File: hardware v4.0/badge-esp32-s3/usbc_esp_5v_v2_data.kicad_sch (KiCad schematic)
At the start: 22 parts, among them J2 Connector, USB-TYPE-C-16P, Q10 AO3424, U11 SY6288F1ABC, U12 SY6288F1ABC, U8 TUSB321AIRWBR

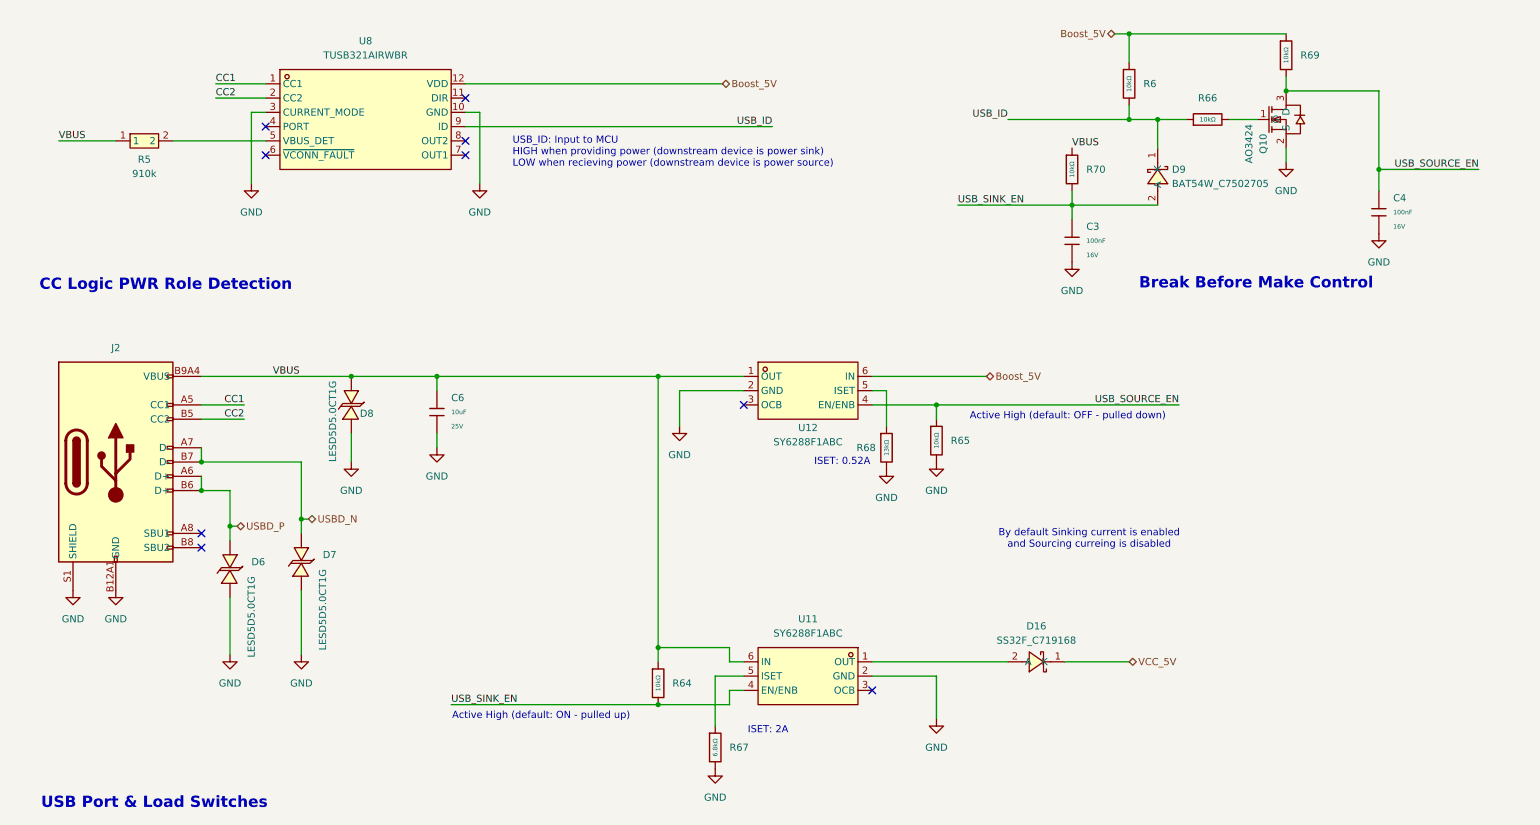
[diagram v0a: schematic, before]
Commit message: finished schematics and layout
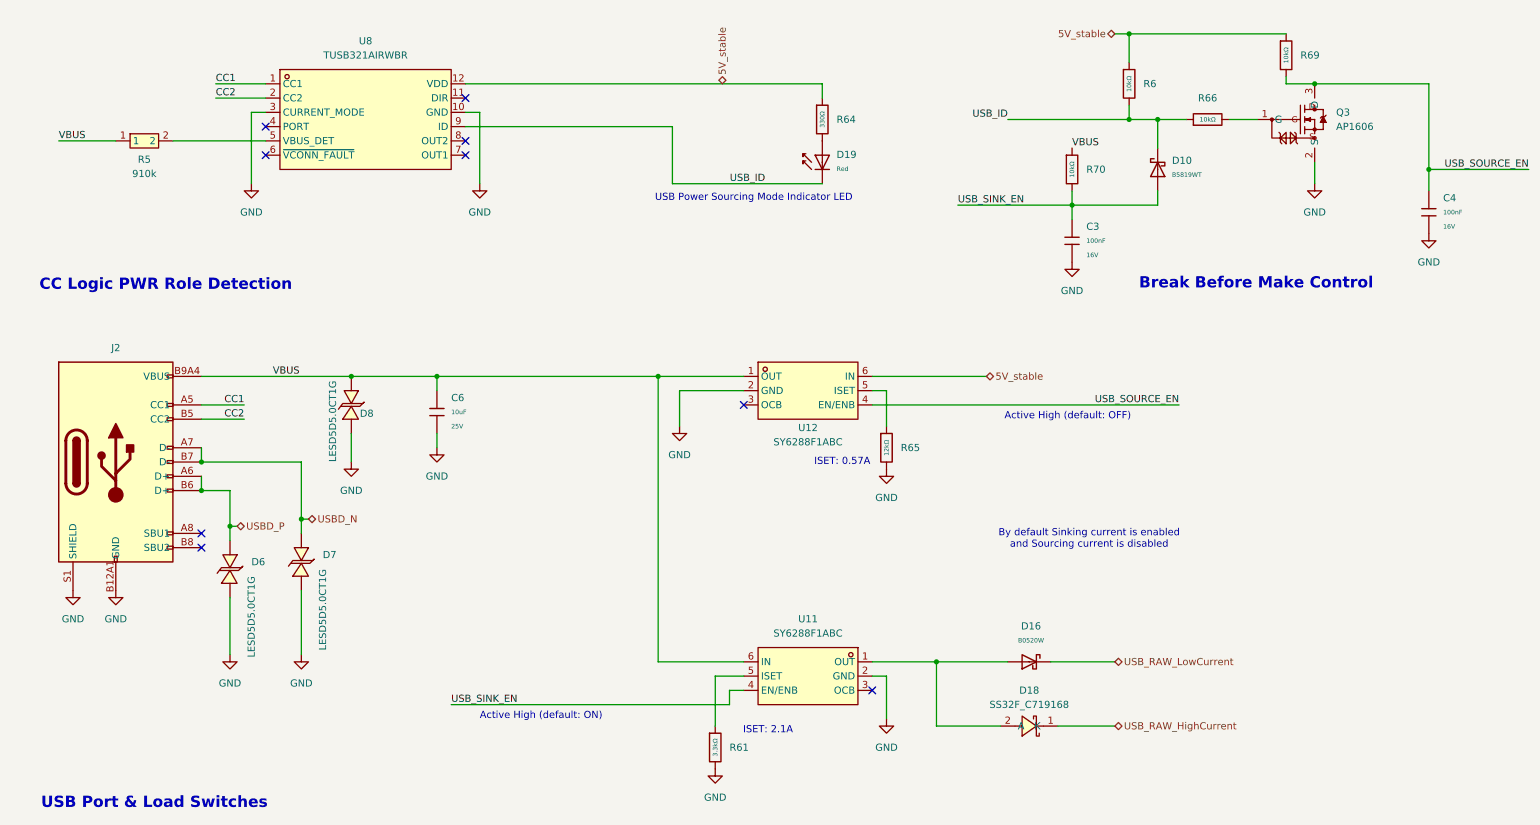
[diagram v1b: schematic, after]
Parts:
- removed D16: SS32F_C719168, lcsc-lib:SMAF_L3.5-W2.6-LS4.7-RD, symbol lcsc-lib:SS32F_C719168
- removed D9: BAT54W_C7502705, lcsc-lib:SOD-123_L2.7-W1.6-LS3.7-RD, symbol lcsc-lib:BAT54W_C7502705
- removed Q10: AO3424, lcsc-lib:SC-59-3_L2.9-W1.6-P0.95-LS2.9-BR, symbol lcsc-lib:AO3424
- removed R64, R65: 10kΩ, PCM_JLCPCB:R_0402, symbol PCM_JLCPCB-Resistors:0402,10kΩ
- removed R67: 6.8kΩ, PCM_JLCPCB:R_0402, symbol PCM_JLCPCB-Resistors:0402,6.8kΩ
- removed R68: 13kΩ, PCM_JLCPCB:R_0603, symbol PCM_JLCPCB-Resistors:0603,13kΩ
- added D10: B5819WT, PCM_JLCPCB:D_SOD-523, symbol PCM_JLCPCB-Diodes:Schottky,B5819WT
- added D16: B0520W, PCM_JLCPCB:D_SOD-123, symbol PCM_JLCPCB-Diodes:Schottky,B0520W
- added D18: SS32F_C719168, lcsc-lib:SMAF_L3.5-W2.6-LS4.7-RD, symbol lcsc-lib:SS32F_C719168
- added D19: Red, PCM_JLCPCB:D_0603, symbol PCM_JLCPCB-Diodes:LED,0603,Red
- added Q3: AP1606, lcsc-lib:DFN-3L_L1.0-W0.6-P0.65-BR, symbol lcsc-lib:AP1606
- added R61: 3.3kΩ, PCM_JLCPCB:R_0402, symbol PCM_JLCPCB-Resistors:0402,3.3kΩ
- added R64: 330Ω, PCM_JLCPCB:R_0402, symbol PCM_JLCPCB-Resistors:0402,330Ω
- added R65: 12kΩ, PCM_JLCPCB:R_0402, symbol PCM_JLCPCB-Resistors:0402,12kΩ
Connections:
- net GND: now also Q3.2 (S), R61.2, R65.2
- net USB_ID: now also D10.1, D19.1
- net USB_SINK_EN: now also D10.2
- net USB_SOURCE_EN: now also Q3.3 (D)
- net at U11.1 (OUT): now also D16.2, D18.2 (A)
- net at U11.5 (ISET): now also R61.1
- net at R66.2: now also Q3.1 (G)
- net at U12.5 (ISET): now also R65.1
- net Boost_5V renamed 5V_stable
- net 5V_stable: now also R64.1
- new net: D19.2, R64.2
- new net USB_RAW_HighCurrent: D18.1 (K)
- new net USB_RAW_LowCurrent: D16.1
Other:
- note added: "Active High (default: OFF)"
- note added: "Active High (default: ON)"
- note added: "By default Sinking current is enabled and Sourcing current is disabled"
- note added: "ISET: 0.57A"
- note added: "ISET: 2.1A"
- note added: "USB Power Sourcing Mode Indicator LED"
- note removed: "Active High (default: OFF - pulled down)"
- note removed: "Active High (default: ON - pulled up)"
- note removed: "By default Sinking current is enabled and Sourcing curreing is disabled"
- note removed: "ISET: 0.52A"
- note removed: "ISET: 2A"
- note removed: "USB_ID: Input to MCU HIGH when providing power (downstream device is power sink) LOW when recieving power (downstream device is power source)"
- moved on the sheet: C4
